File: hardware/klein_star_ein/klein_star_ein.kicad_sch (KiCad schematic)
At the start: 31 parts, among them U1 ECP5UM25, U2 MT41K512M16, U3 MT41K512M16

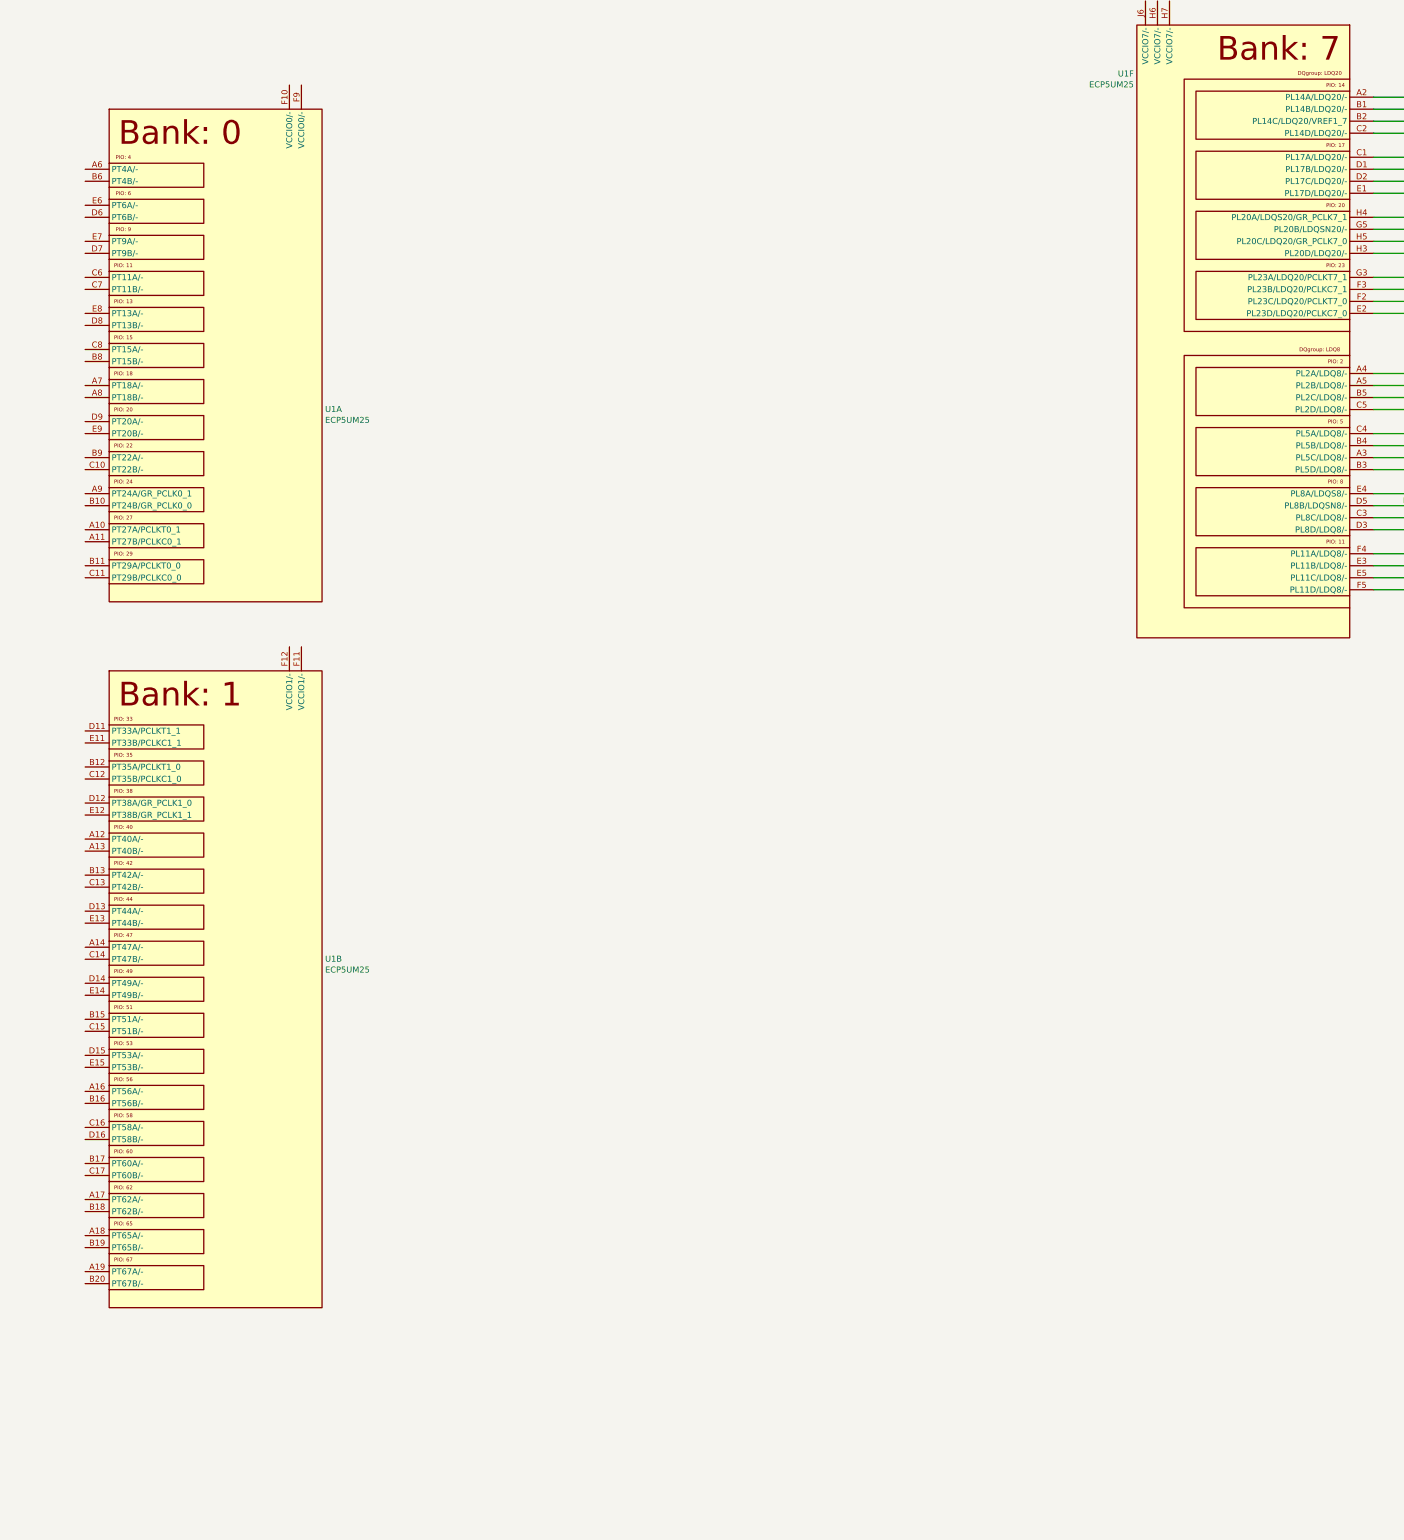
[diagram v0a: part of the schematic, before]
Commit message: no idea what's here
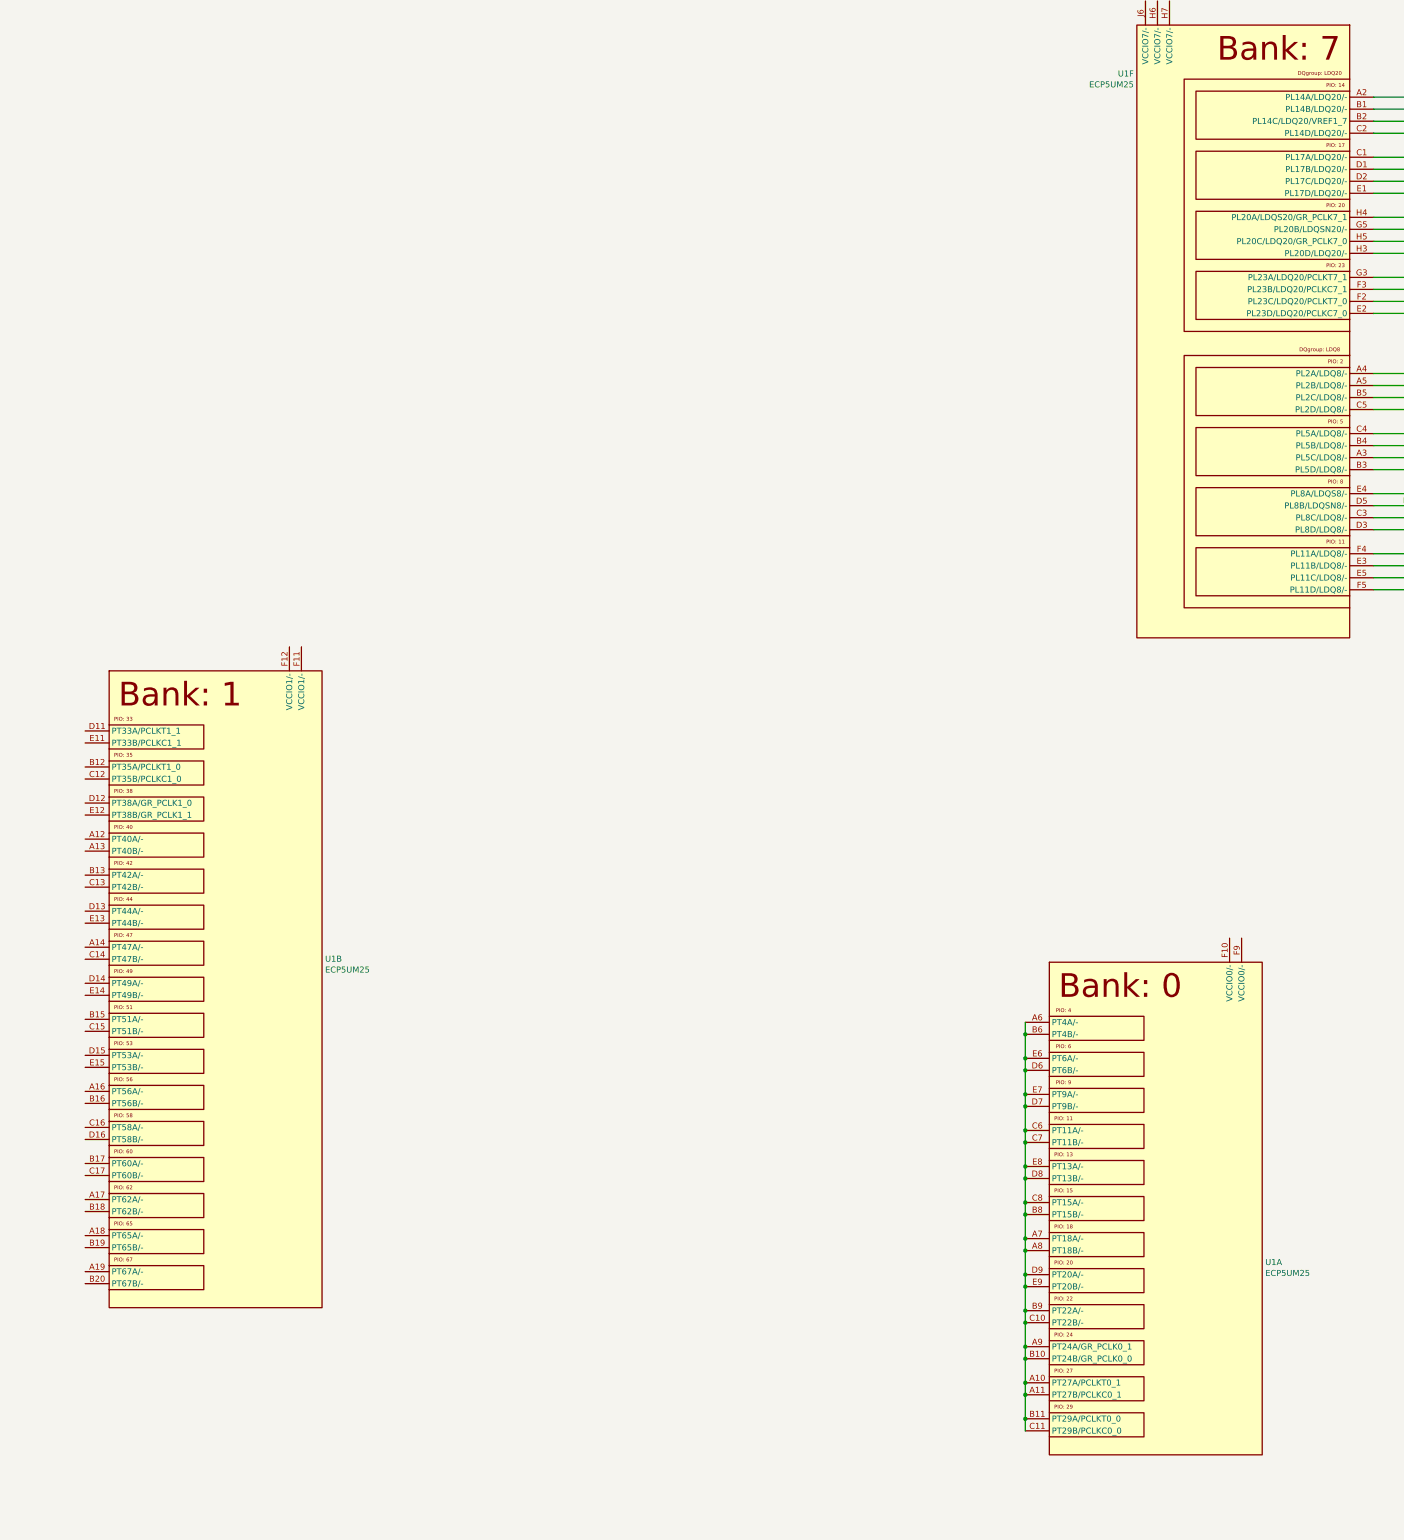
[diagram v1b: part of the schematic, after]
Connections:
- net at U1.A10 (PT27A/PCLKT0_1): now also U1.A11 (PT27B/PCLKC0_1), U1.A6 (PT4A/-), U1.A7 (PT18A/-), U1.A8 (PT18B/-), U1.A9 (PT24A/GR_PCLK0_1), U1.B10 (PT24B/GR_PCLK0_0), U1.B11 (PT29A/PCLKT0_0), U1.B6 (PT4B/-), U1.B8 (PT15B/-), U1.B9 (PT22A/-), U1.C10 (PT22B/-), U1.C11 (PT29B/PCLKC0_0), U1.C6 (PT11A/-), U1.C7 (PT11B/-), U1.C8 (PT15A/-), U1.D6 (PT6B/-), U1.D7 (PT9B/-), U1.D8 (PT13B/-), U1.D9 (PT20A/-), U1.E6 (PT6A/-), U1.E7 (PT9A/-), U1.E8 (PT13A/-), U1.E9 (PT20B/-)
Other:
- moved on the sheet: U1A
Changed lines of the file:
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@@
 (kicad_sch (version 20201015) (generator eeschema)
   (paper "A0")
+  (junction (at 648.97 266.7) (diameter 0.9144) (color 0 0 0 0))
+  (junction (at 648.97 271.78) (diameter 0.9144) (color 0 0 0 0))
+  (junction (at 648.97 274.32) (diameter 0.9144) (color 0 0 0 0))
+  (junction (at 648.97 279.4) (diameter 0.9144) (color 0 0 0 0))
+  (junction (at 648.97 281.94) (diameter 0.9144) (color 0 0 0 0))
+  (junction (at 648.97 287.02) (diameter 0.9144) (color 0 0 0 0))
+  (junction (at 648.97 289.56) (diameter 0.9144) (color 0 0 0 0))
+  (junction (at 648.97 294.64) (diameter 0.9144) (color 0 0 0 0))
+  (junction (at 648.97 297.18) (diameter 0.9144) (color 0 0 0 0))
+  (junction (at 648.97 302.26) (diameter 0.9144) (color 0 0 0 0))
+  (junction (at 648.97 304.8) (diameter 0.9144) (color 0 0 0 0))
+  (junction (at 648.97 309.88) (diameter 0.9144) (color 0 0 0 0))
+  (junction (at 648.97 312.42) (diameter 0.9144) (color 0 0 0 0))
+  (junction (at 648.97 317.5) (diameter 0.9144) (color 0 0 0 0))
+  (junction (at 648.97 320.04) (diameter 0.9144) (color 0 0 0 0))
+  (junction (at 648.97 325.12) (diameter 0.9144) (color 0 0 0 0))
+  (junction (at 648.97 327.66) (diameter 0.9144) (color 0 0 0 0))
+  (junction (at 648.97 332.74) (diameter 0.9144) (color 0 0 0 0))
+  (junction (at 648.97 335.28) (diameter 0.9144) (color 0 0 0 0))
+  (junction (at 648.97 340.36) (diameter 0.9144) (color 0 0 0 0))
+  (junction (at 648.97 342.9) (diameter 0.9144) (color 0 0 0 0))
+  (junction (at 648.97 347.98) (diameter 0.9144) (color 0 0 0 0))
   (junction (at 833.12 161.29) (diameter 0.9144) (color 0 0 0 0))
   (junction (at 833.12 163.83) (diameter 0.9144) (color 0 0 0 0))
@@
   (junction (at 1161.415 77.47) (diameter 0.9144) (color 0 0 0 0))
   (junction (at 1162.685 151.765) (diameter 0.9144) (color 0 0 0 0))
-  (no_connect (at 1066.8 572.77))
+  (no_connect (at 1066.8 570.23))
+  (no_connect (at 1066.8 539.75))
+  (no_connect (at 1066.8 560.07))
+  (no_connect (at 1066.8 529.59))
+  (no_connect (at 1066.8 519.43))
+  (no_connect (at 1066.8 527.05))
+  (no_connect (at 1066.8 542.29))
+  (no_connect (at 1066.8 532.13))
+  (no_connect (at 1066.8 575.31))
+  (no_connect (at 1066.8 521.97))
   (no_connect (at 1066.8 544.83))
+  (no_connect (at 1066.8 562.61))
+  (no_connect (at 1066.8 549.91))
+  (no_connect (at 1066.8 557.53))
+  (no_connect (at 1066.8 582.93))
+  (no_connect (at 1066.8 577.85))
   (no_connect (at 1066.8 565.15))
   (no_connect (at 1066.8 524.51))
-  (no_connect (at 1066.8 577.85))
-  (no_connect (at 1066.8 560.07))
-  (no_connect (at 1066.8 562.61))
-  (no_connect (at 1066.8 542.29))
-  (no_connect (at 1066.8 570.23))
-  (no_connect (at 1066.8 529.59))
+  (no_connect (at 1066.8 554.99))
   (no_connect (at 1066.8 567.69))
-  (no_connect (at 1066.8 532.13))
-  (no_connect (at 1066.8 549.91))
-  (no_connect (at 1066.8 519.43))
+  (no_connect (at 1066.8 547.37))
+  (no_connect (at 1066.8 534.67))
   (no_connect (at 1066.8 537.21))
   (no_connect (at 1066.8 552.45))
-  (no_connect (at 1066.8 557.53))
-  (no_connect (at 1066.8 534.67))
-  (no_connect (at 1066.8 575.31))
-  (no_connect (at 1066.8 521.97))
+  (no_connect (at 1066.8 572.77))
   (no_connect (at 1066.8 580.39))
-  (no_connect (at 1066.8 554.99))
-  (no_connect (at 1066.8 582.93))
-  (no_connect (at 1066.8 547.37))
-  (no_connect (at 1066.8 539.75))
-  (no_connect (at 1066.8 527.05))
+  (wire (pts (xy 648.97 264.16) (xy 648.97 266.7))
+    (stroke (width 0) (type solid) (color 0 0 0 0))
+  )
+  (wire (pts (xy 648.97 266.7) (xy 648.97 271.78))
+    (stroke (width 0) (type solid) (color 0 0 0 0))
+  )
+  (wire (pts (xy 648.97 271.78) (xy 648.97 274.32))
+    (stroke (width 0) (type solid) (color 0 0 0 0))
+  )
+  (wire (pts (xy 648.97 274.32) (xy 648.97 279.4))
+    (stroke (width 0) (type solid) (color 0 0 0 0))
+  )
+  (wire (pts (xy 648.97 279.4) (xy 648.97 281.94))
+    (stroke (width 0) (type solid) (color 0 0 0 0))
+  )
+  (wire (pts (xy 648.97 281.94) (xy 648.97 287.02))
+    (stroke (width 0) (type solid) (color 0 0 0 0))
+  )
+  (wire (pts (xy 648.97 287.02) (xy 648.97 289.56))
+    (stroke (width 0) (type solid) (color 0 0 0 0))
+  )
+  (wire (pts (xy 648.97 289.56) (xy 648.97 294.64))
+    (stroke (width 0) (type solid) (color 0 0 0 0))
+  )
+  (wire (pts (xy 648.97 294.64) (xy 648.97 297.18))
+    (stroke (width 0) (type solid) (color 0 0 0 0))
+  )
+  (wire (pts (xy 648.97 297.18) (xy 648.97 302.26))
+    (stroke (width 0) (type solid) (color 0 0 0 0))
+  )
+  (wire (pts (xy 648.97 302.26) (xy 648.97 304.8))
+    (stroke (width 0) (type solid) (color 0 0 0 0))
+  )
+  (wire (pts (xy 648.97 304.8) (xy 648.97 309.88))
+    (stroke (width 0) (type solid) (color 0 0 0 0))
+  )
+  (wire (pts (xy 648.97 309.88) (xy 648.97 312.42))
+    (stroke (width 0) (type solid) (color 0 0 0 0))
+  )
+  (wire (pts (xy 648.97 312.42) (xy 648.97 317.5))
+    (stroke (width 0) (type solid) (color 0 0 0 0))
+  )
+  (wire (pts (xy 648.97 317.5) (xy 648.97 320.04))
+    (stroke (width 0) (type solid) (color 0 0 0 0))
+  )
+  (wire (pts (xy 648.97 320.04) (xy 648.97 325.12))
+    (stroke (width 0) (type solid) (color 0 0 0 0))
+  )
+  (wire (pts (xy 648.97 325.12) (xy 648.97 327.66))
+    (stroke (width 0) (type solid) (color 0 0 0 0))
+  )
+  (wire (pts (xy 648.97 327.66) (xy 648.97 332.74))
+    (stroke (width 0) (type solid) (color 0 0 0 0))
+  )
+  (wire (pts (xy 648.97 332.74) (xy 648.97 335.28))
+    (stroke (width 0) (type solid) (color 0 0 0 0))
+  )
+  (wire (pts (xy 648.97 335.28) (xy 648.97 340.36))
+    (stroke (width 0) (type solid) (color 0 0 0 0))
+  )
+  (wire (pts (xy 648.97 340.36) (xy 648.97 342.9))
+    (stroke (width 0) (type solid) (color 0 0 0 0))
+  )
+  (wire (pts (xy 648.97 342.9) (xy 648.97 347.98))
+    (stroke (width 0) (type solid) (color 0 0 0 0))
+  )
+  (wire (pts (xy 648.97 347.98) (xy 648.97 350.52))
+    (stroke (width 0) (type solid) (color 0 0 0 0))
+  )
   (wire (pts (xy 722.63 76.2) (xy 744.22 76.2))
     (stroke (width 0) (type solid) (color 0 0 0 0))
@@
     )
   )
-  (symbol (lib_name "ECP5UM25:ECP5UM25_8") (lib_id "ECP5UM25:ECP5UM25") (at 455.295 71.12 0) (unit 1)
-    (in_bom yes) (on_board yes)
-    (property "Reference" "U1" (id 0) (at 500.9306 134.5503 0)
-      (effects (font (size 1.27 1.27)) (justify left))
-    )
-    (property "Value" "ECP5UM25" (id 1) (at 500.9306 136.849 0)
-      (effects (font (size 1.27 1.27)) (justify left))
-    )
-    (property "Footprint" "Package_BGA:Lattice_caBGA-381_17.0x17.0mm_Layout20x20_P0.8mm_Ball0.4mm_Pad0.4mm_NSMD" (id 2) (at 455.295 63.12 0)
-      (effects (font (size 1.27 1.27)) hide)
-    )
-    (property "Datasheet" "" (id 3) (at 455.295 71.12 0)
-      (effects (font (size 1.27 1.27)) hide)
-    )
+  (symbol (lib_name "ECP5UM25:ECP5UM25_8") (lib_id "ECP5UM25:ECP5UM25") (at 654.05 251.46 0) (unit 1)
+    (in_bom yes) (on_board yes)
+    (property "Reference" "U1" (id 0) (at 699.6856 314.8903 0)
+      (effects (font (size 1.27 1.27)) (justify left))
+    )
+    (property "Value" "ECP5UM25" (id 1) (at 699.6856 317.189 0)
+      (effects (font (size 1.27 1.27)) (justify left))
+    )
+    (property "Footprint" "Package_BGA:Lattice_caBGA-381_17.0x17.0mm_Layout20x20_P0.8mm_Ball0.4mm_Pad0.4mm_NSMD" (id 2) (at 654.05 243.46 0)
+      (effects (font (size 1.27 1.27)) hide)
+    )
+    (property "Datasheet" "" (id 3) (at 654.05 251.46 0)
+      (effects (font (size 1.27 1.27)) hide)
+    )
